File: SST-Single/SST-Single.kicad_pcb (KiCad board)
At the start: 2 copper layers, 45 x 36 mm, 16 parts, among them J1 Conn_01x03_Pin, J2 Conn_01x04_Pin, J3 MJ-179PH, SW1 EDS102SZ, U1 FT231XS-Breakout, U2 LT1785AxN8

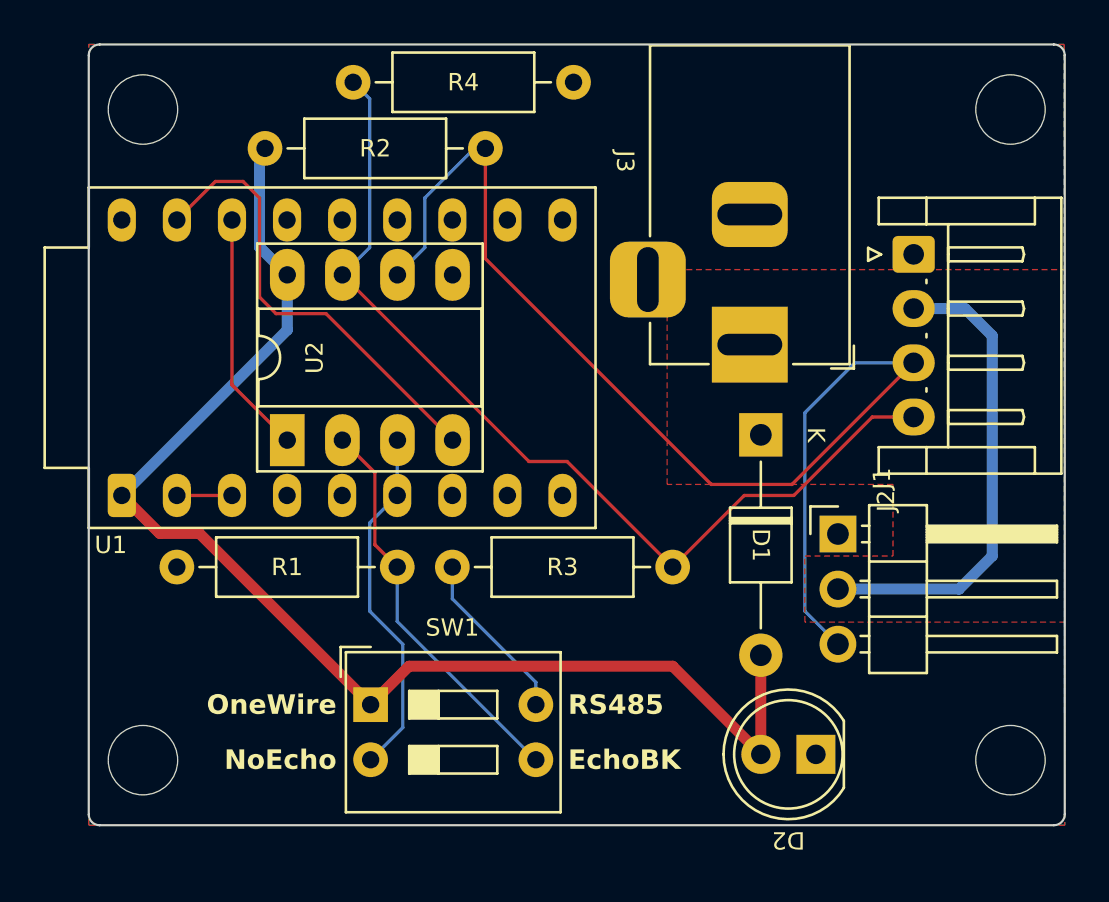
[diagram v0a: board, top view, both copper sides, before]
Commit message: Update PCB pattern
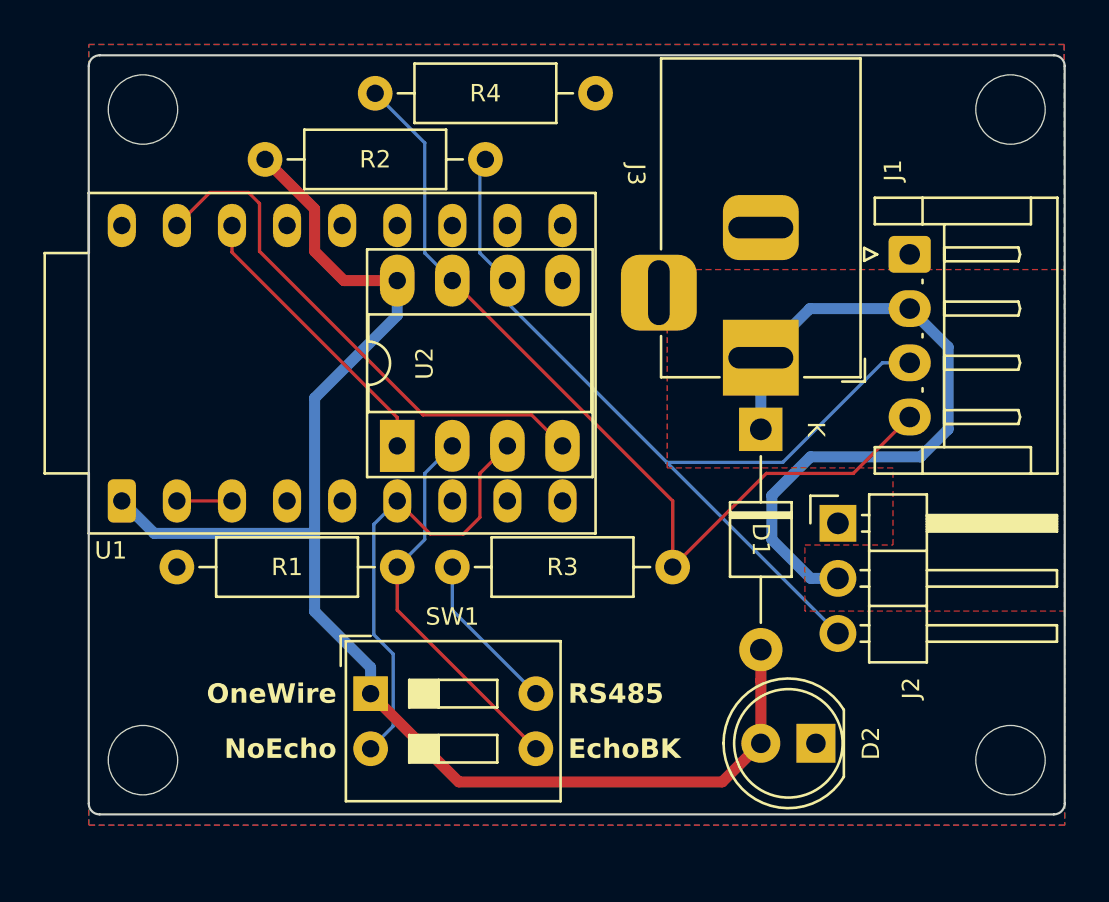
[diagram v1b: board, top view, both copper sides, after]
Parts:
- moved U2 5.08 mm to (114.2, 62.5)
- moved R4 1.14 mm to (123.4, 46.3)
- moved J3 0.79 mm to (131.0, 58.4)
- moved D2 0.51 mm to (133.5, 76.2)
- moved R2 0.51 mm to (118.3, 49.3)
- moved SW1 0.51 mm to (113.0, 73.9)
- moved J1 0.49 mm to (134.5, 66.1)
- moved D1 0.25 mm to (131.0, 61.7)
- moved U1 0.25 mm to (111.7, 58.7)
- moved J2 0.18 mm to (137.9, 53.7)
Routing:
- net /RS485A: track 56.5 -> 41.9 mm
- net VCC: track 22.0 -> 32.6 mm
- net +5V: track 60.2 -> 65.5 mm
- net /RXDEN: track 16.5 -> 21.3 mm
- net /TXD: track 21.1 -> 24.5 mm
- net /RS485B: track 44.5 -> 41.3 mm
- net /RXD: track 11.2 -> 13.3 mm
- net /~{RS485_RE}: track 18.4 -> 17.7 mm
- net /RS485B_UP: track 7.94 -> 7.43 mm
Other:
- board size 45 x 36 mm -> 45 x 35 mm
